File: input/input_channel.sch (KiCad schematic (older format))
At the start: 0 parts

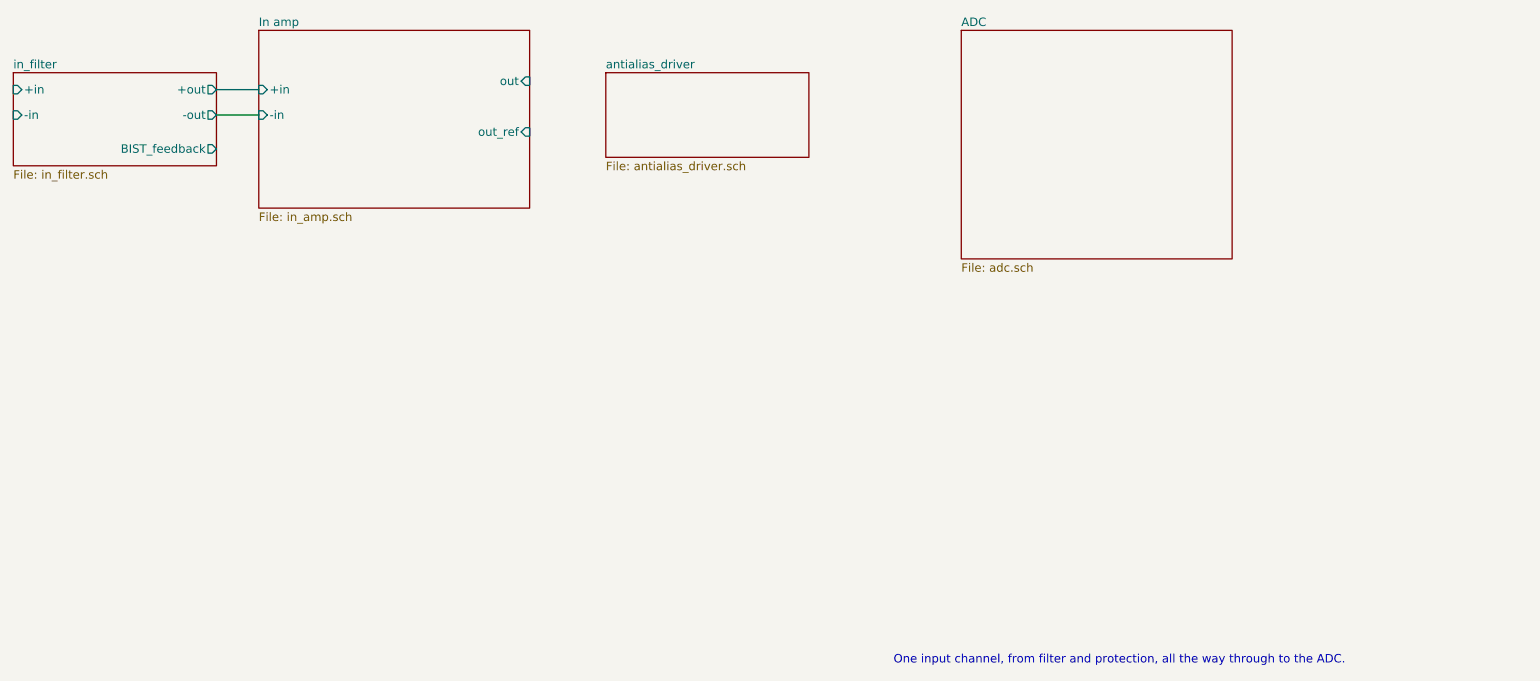
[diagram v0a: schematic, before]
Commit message: More work on input board
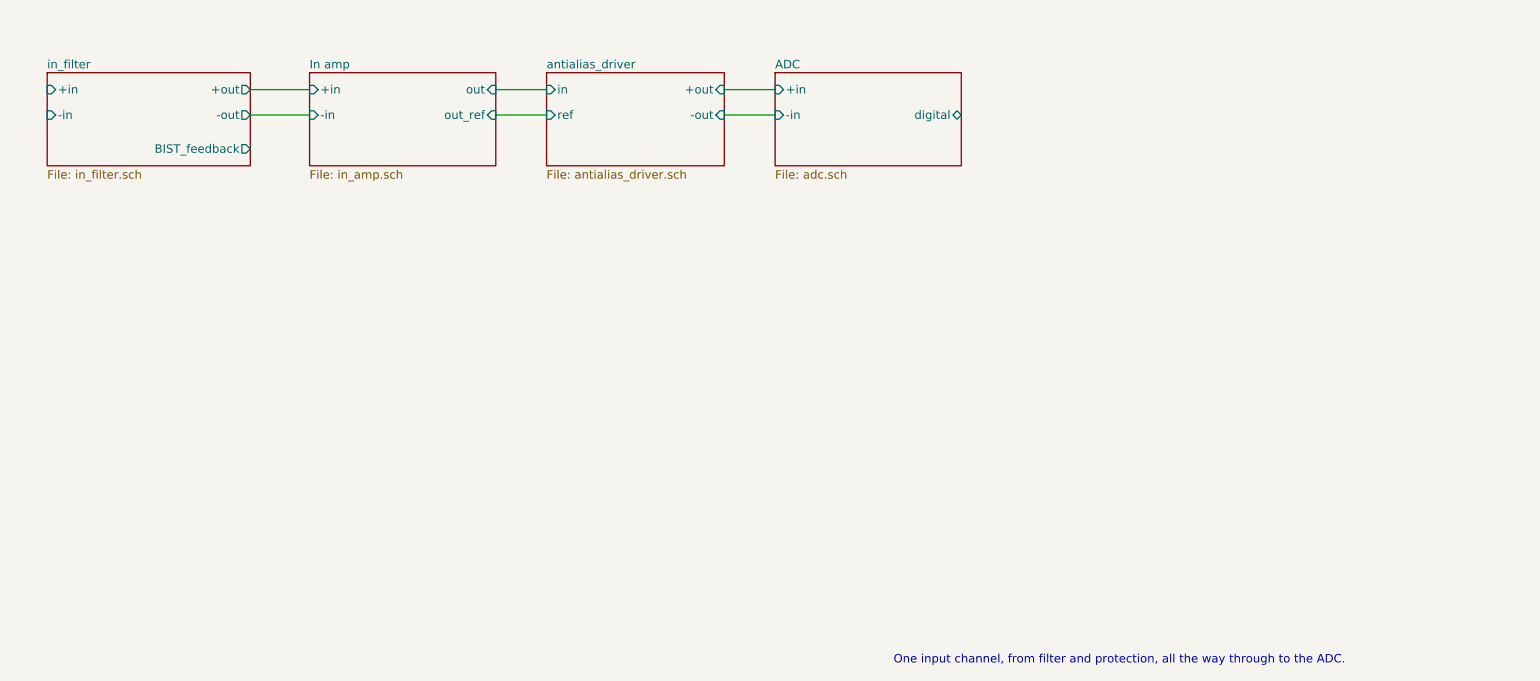
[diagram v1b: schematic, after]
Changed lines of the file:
@@
 $EndDescr
 $Sheet
-S 7550 3000 1600 1350
+S 6450 3250 1100 550
 U 5DA78AA2
 F0 "ADC" 50
 F1 "adc.sch" 50
+F2 "+in" I L 6450 3350 50
+F3 "-in" I L 6450 3500 50
+F4 "digital" B R 7550 3500 50
 $EndSheet
-Wire Wire Line
-	3150 3350 3400 3350
 $Sheet
-S 5450 3250 1200 500
+S 5100 3250 1050 550
 U 5DE6CDF8
 F0 "antialias_driver" 50
 F1 "antialias_driver.sch" 50
+F2 "in" I L 5100 3350 50
+F3 "-out" I R 6150 3500 50
+F4 "+out" I R 6150 3350 50
+F5 "ref" I L 5100 3500 50
 $EndSheet
 Text Notes 7150 6750 0    50   ~ 0
 One input channel, from filter and protection, all the way through to the ADC.
-Wire Wire Line
-	3150 3500 3400 3500
 $Sheet
-S 1950 3250 1200 550
+S 2150 3250 1200 550
 U 5DE42731
 F0 "in_filter" 50
 F1 "in_filter.sch" 50
-F2 "+out" O R 3150 3350 50
-F3 "-out" O R 3150 3500 50
-F4 "-in" I L 1950 3500 50
-F5 "+in" I L 1950 3350 50
-F6 "BIST_feedback" O R 3150 3700 50
+F2 "+out" O R 3350 3350 50
+F3 "-out" O R 3350 3500 50
+F4 "-in" I L 2150 3500 50
+F5 "+in" I L 2150 3350 50
+F6 "BIST_feedback" O R 3350 3700 50
 $EndSheet
 $Sheet
-S 3400 3000 1600 1050
+S 3700 3250 1100 550
 U 5DA78BF5
 F0 "In amp" 50
 F1 "in_amp.sch" 50
-F2 "-in" I L 3400 3500 50
-F3 "+in" I L 3400 3350 50
-F4 "out" I R 5000 3300 50
-F5 "out_ref" I R 5000 3600 50
+F2 "-in" I L 3700 3500 50
+F3 "+in" I L 3700 3350 50
+F4 "out" I R 4800 3350 50
+F5 "out_ref" I R 4800 3500 50
 $EndSheet
+Wire Wire Line
+	4800 3350 5100 3350
+Wire Wire Line
+	4800 3500 5100 3500
+Wire Wire Line
+	6150 3500 6450 3500
+Wire Wire Line
+	6150 3350 6450 3350
+Wire Wire Line
+	3350 3350 3700 3350
+Wire Wire Line
+	3350 3500 3700 3500
 $EndSCHEMATC
